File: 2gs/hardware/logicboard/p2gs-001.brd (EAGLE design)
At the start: 91 x 90 mm, 66 parts, among them J1 MKR, J10 1-Wire, J2 GPIO, J3 Vcc, J5 SPI, J6 LED, J7 DIN5, K1 G5V1, Q1 220mA/50V/3.5Ω, Q2 220mA/50V/3.5Ω, T1 2SC1815

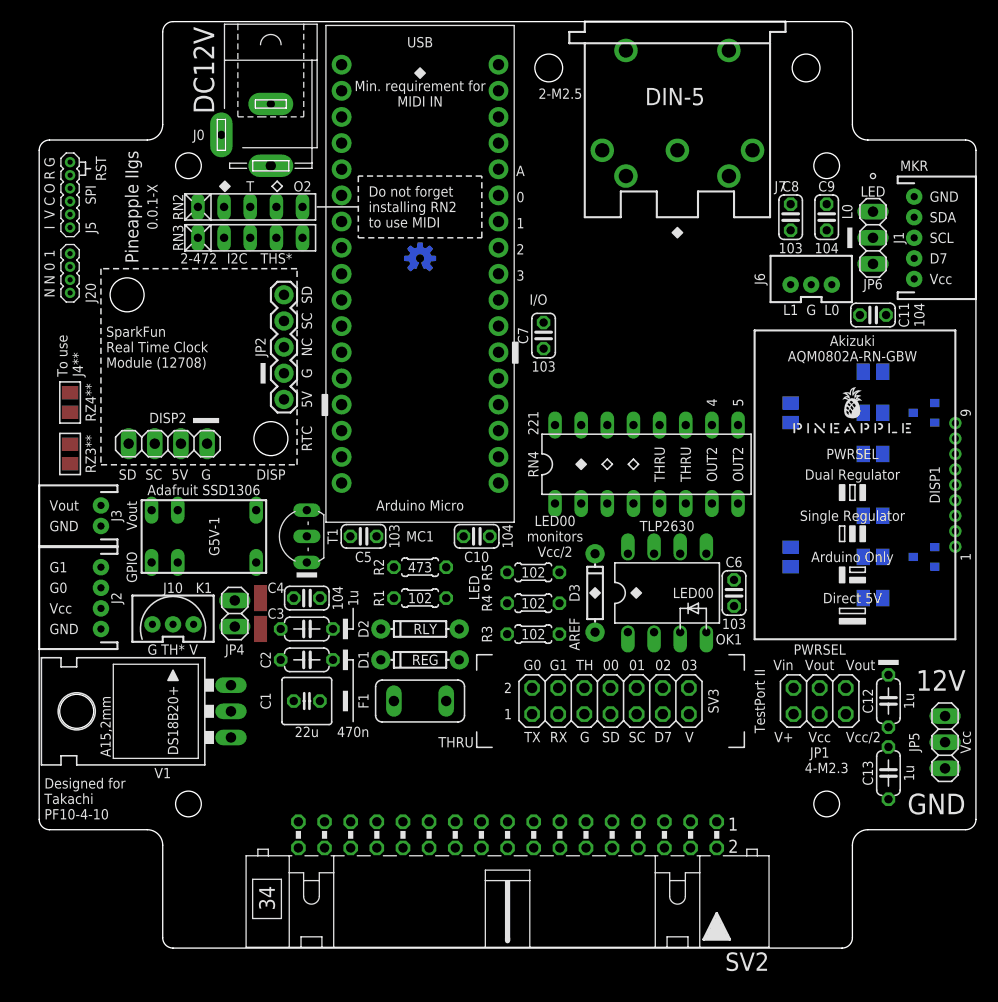
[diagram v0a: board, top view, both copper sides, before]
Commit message: Routed.
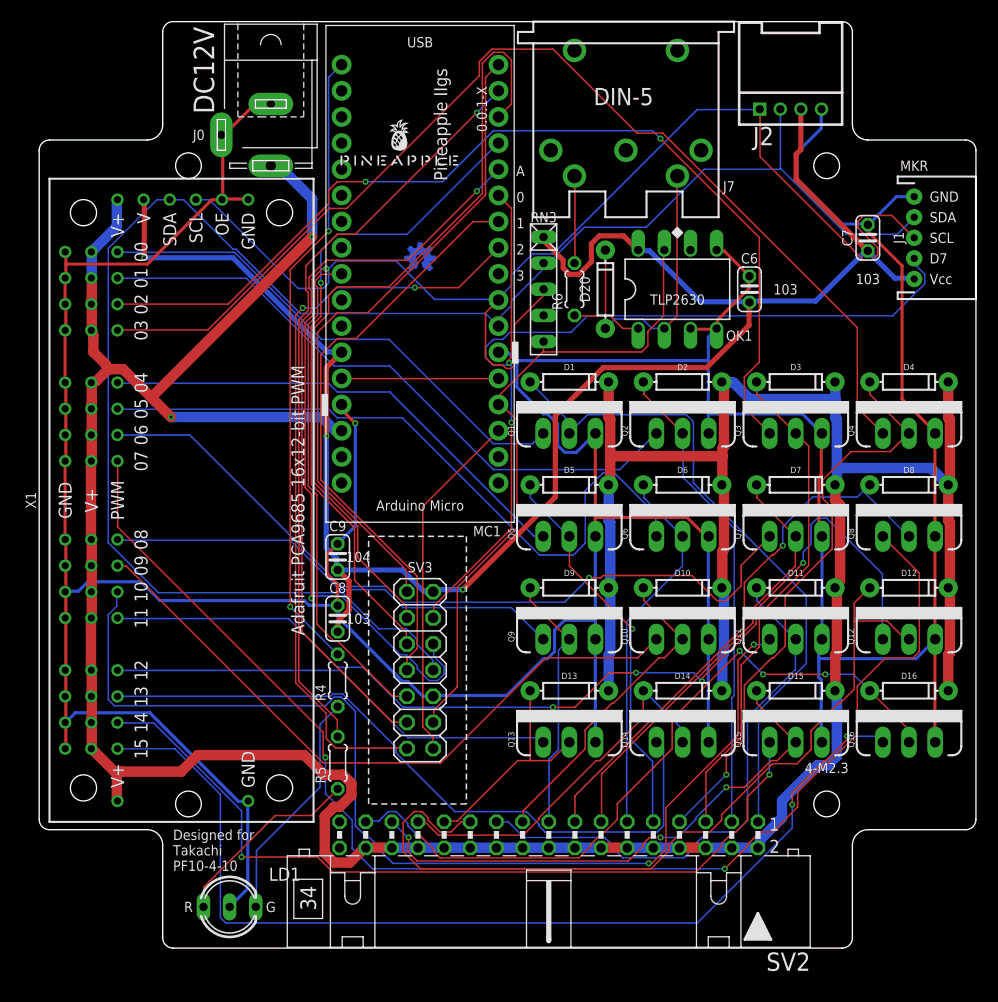
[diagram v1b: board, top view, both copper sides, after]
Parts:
- removed A, B: (no value), wirepad:SMD1,27-2,54
- removed C1: 22u, rcl:C025-050X050
- removed C10, C11, C4: 100n, rcl:C025-024X044
- removed C12, C13, C3: 1u, rcl:C050-024X044
- removed C2: 470n, rcl:C050-024X044
- removed C5: 10n, resistor:C025-024X044
- removed DISP1: AQM0802A-RN-GBW, AQM0802A-RN-GBW:AQM0802A-RN-GBW-FOOTPRINT
- removed DISP2: MNTR, pinhead:1X04
- removed F1: 1.8A, fuse:TE5
- removed H1, H2: STAND-OFF, SparkFun-Hardware:STAND-OFF
- removed J10: 1-Wire, SparkFun-Connectors:JST-3-PTH-VERT
- removed J20: (no value), SparkFun-Connectors:1X04_1.27MM
- removed J3: Vcc, SparkFun-Connectors:JST-2-PTH
- removed J5: SPI, SparkFun-Connectors:1X06_1.27MM
- removed J6: LED, SparkFun-Connectors:JST-3-PTH-VERT
- removed JP1: PWRSEL, pinhead:2X03
- removed JP2: RTC, SparkFun-Connectors:1X05
- removed JP4: RLYJMP, pinhead:1X02
- removed JP5: PWR, pinhead:1X03
- removed JP6: LED, pinhead:1X03
- removed K1: G5V1, relay:G5V1
- removed R1, R3: 1k, resistor:0204/5
- removed R101, R102, R103, R104: 10k, rcl:M2012
- removed R2: 47k, resistor:0204/5
- removed RN2: 4.7k, resistor-net:RN-5
- removed RN4: 220, resistor-dil:DIL16
- removed RZ1***, RZ2***, RZ3**, RZ4**, VCCBRIDGE***: Inf, rcl:M2012
- removed T1: 2SC1815, transistor:TO92-ECB
- removed V1: 5V, v-reg:78XXL
- removed VDDBRIDGE: 0, rcl:M2012
- added D10, D11, D12, D13, D14, D15, D16, D4, D5, D6, D7, D8, D9: 200mA/100V/1V, SparkFun-DiscreteSemi:DIODE-1N4148
- added D20: (no value), SparkFun-DiscreteSemi:DIODE-1N4148
- added LD1: Red/Green, led:DUOLED-C-5MM
- added Q10, Q11, Q12, Q13, Q14, Q15, Q16, Q3, Q4, Q5, Q6, Q7, Q8, Q9: 60V/32A/35mΩ, SparkFun-DiscreteSemi:TO220V
- added R6: 220, resistor:0204/5
- added X1: ADAFRUIT-PCA9685, adafruit-pca9685:ADAFRUIT-PCA9685-FOOTPRINT
- D1, D2, D3: value (none) -> 200mA/100V/1V
- J0: value (none) -> 12V
- J2: value GPIO -> (none); device SparkFun-Connectors:JST-4-PTH -> Connector:4P-2.0-90D
- Q1, Q2: value 220mA/50V/3.5Ω -> 60V/32A/35mΩ; device SparkFun-DiscreteSemi:SOT23-3 -> SparkFun-DiscreteSemi:TO220V
- R4, R5: value 1k -> 330
- SV2: value (none) -> LD
- moved J2 82.1 mm to (73.0, 81.5), turned to 0 degrees
- moved C8 58.8 mm to (29.0, 32.0)
- moved C9 57.8 mm to (29.0, 38.0)
- moved U$1 51.1 mm to (35.0, 76.0)
- moved Q1 36.5 mm to (51.5, 50.0), flipped to the top, turned to 0 degrees
- moved D2 35.0 mm to (62.5, 55.0), turned to 0 degrees
- moved C7 32.9 mm to (80.5, 69.0)
- moved D1 30.6 mm to (51.5, 55.0), turned to 0 degrees
- moved C6 29.5 mm to (69.0, 64.0)
- moved OK1 29.5 mm to (62.0, 64.0)
- moved RN3 28.9 mm to (49.0, 64.0), turned to 270 degrees
- moved D3 28.3 mm to (73.5, 55.0), turned to 0 degrees
- moved R5 26.5 mm to (29.0, 18.0), turned to 90 degrees
- moved Q2 23.6 mm to (62.5, 50.0), flipped to the top, turned to 0 degrees
- moved R4 20.4 mm to (29.0, 26.0), turned to 90 degrees
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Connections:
- removed net CAP1N: C12.2, DISP1.3
- removed net CAP1P: C12.1, DISP1.4
- removed net LCDVOUT: C13.2, DISP1.2
- removed net MNTRA: OK1.4, RN4.16
- removed net NMO2RTN: RN2.5
- removed net NMORTN: RN2.4
- removed net NMTRTN: RN2.3
- removed net RLYDRV: R1.1, R2.2, T1.B
- removed net RLYOUT: K1.10
- removed net RLYOUT1: RZ3**.2
- removed net RLYOUT2: RZ4**.2
- removed net RLYSNK: D2.A, K1.9, T1.C
- removed net SCL3V: DISP1.8, Q1.2, R102.1, RZ1***.2
- removed net SDA3V: DISP1.7, Q2.2, R104.1, RZ2***.2
- removed net V+: C1.1, C2.1, D1.C, J0.3, JP1.1, JP5.3, V1.IN
- removed net VCC/2: JP1.5, R3.2, RN4.1
- removed net VCC/VDD: C11.1, C13.1, DISP1.5, DISP1.9, VCCBRIDGE***.1, VDDBRIDGE.1
- removed net VOUT: F1.2, JP1.4, JP1.6
- removed net VOUTRAW: B.1, C3.1, C4.1, D1.A, J3.2, JP4.2, K1.5, K1.6, RZ3**.1, V1.OUT
- removed net VOUTRAW2: A.1, F1.1, JP4.1, K1.1, RZ4**.1
- new net LD00: D1.A, Q1.2, SV2.1
- new net LD01: D2.A, Q2.2, SV2.3
- new net LD02: D3.A, Q3.2, SV2.5
- new net LD03: D4.A, Q4.2, SV2.7
- new net LD04: D5.A, Q5.2, SV2.9
- new net LD05: D6.A, Q6.2, SV2.11
- new net LD06: D7.A, Q7.2, SV2.13
- new net LD07: D8.A, Q8.2, SV2.15
- new net LD08: D9.A, Q9.2, SV2.17
- new net LD09: D10.A, Q10.2, SV2.19
- new net LD10: D11.A, Q11.2, SV2.21
- new net LD11: D12.A, Q12.2, SV2.23
- new net LD12: D13.A, Q13.2, SV2.25
- new net LD13: D14.A, Q14.2, SV2.27
- new net LD14: D15.A, Q15.2, SV2.29
- new net LD15: D16.A, Q16.2, SV2.31
- new net PWM00: Q1.1, X1.PWM00
- new net PWM01: Q2.1, X1.PWM01
- new net PWM02: Q3.1, X1.PWM02
- new net PWM03: Q4.1, X1.PWM03
- new net PWM04: Q5.1, X1.PWM04
- new net PWM05: Q6.1, X1.PWM05
- new net PWM06: Q7.1, X1.PWM06
- new net PWM07: Q8.1, X1.PWM07
- new net PWM08: Q9.1, X1.PWM08
- new net PWM09: Q10.1, X1.PWM09
- new net PWM10: Q11.1, X1.PWM10
- new net PWM11: Q12.1, X1.PWM11
- new net PWM12: Q13.1, X1.PWM12
- new net PWM13: Q14.1, X1.PWM13
- new net PWM14: Q15.1, X1.PWM14
- new net PWM15: Q16.1, X1.PWM15
- net AREF: no longer C10.1, R3.1
- net GND: now also J2.4, LD1.C, OK1.4, Q1.3, Q10.3, Q11.3, Q12.3, Q13.3, Q14.3, Q15.3, Q16.3, Q2.3, Q3.3, Q4.3, Q5.3, Q6.3, Q7.3, Q8.3, Q9.3, X1.GND00, X1.GND01, X1.GND02, X1.GND03, X1.GND04, X1.GND05, X1.GND06, X1.GND07, X1.GND08, X1.GND09, X1.GND10, X1.GND11, X1.GND12, X1.GND13, X1.GND14, X1.GND15, X1.LGND, X1.LOE, X1.RGND; no longer C1.2, C10.2, C11.2, C2.2, C3.2, C4.2, C5.2, DISP1.6, DISP2.1, J10.1, J2.1, J3.1, J5.6, J6.2, JP2.2, JP5.1, JP6.2, R2.1, T1.E, V1.GND
- net GPIO0: no longer J2.3, J20.3
- net GPIO1: no longer J2.4, J20.4
- net LED0A: now also LD1.AR; no longer J6.3, JP6.3
- net LED1A: now also LD1.AX; no longer J6.1, JP6.1
- net MIDIINSND: now also D20.C, R6.1; no longer D3.C, RN4.2
- net MIRTN: now also D20.A; no longer D3.A
- net MISND: now also R6.2; no longer RN4.15
- net MISO: no longer J5.1
- net MNTR: no longer OK1.6, RN3.5
- net MOSI: no longer J5.4
- net RLY: no longer R1.2
- net RST: no longer J5.5
- net RX: now also RN3.5; no longer RN2.2
- net SCK: no longer J5.3
- net SCL: now also J2.1, X1.LSCL; no longer DISP2.3, JP2.4, Q1.3, R101.1, RZ1***.1
- net SDA: now also J2.2, X1.LSDA; no longer DISP2.4, JP2.5, Q2.3, R103.1, RZ2***.1
- net THS: no longer J10.2, RN3.4
- net VCC: now also J2.3, X1.LVCC; no longer C5.1, D2.C, DISP2.2, J10.3, J2.2, J5.2, JP1.3, JP2.1, JP5.2, K1.2, R101.2, R103.2, RN2.1, VCCBRIDGE***.2
- net VDD: no longer Q1.1, Q2.1, R102.2, R104.2, VDDBRIDGE.2
- net VIN: now also D1.C, D10.C, D11.C, D12.C, D13.C, D14.C, D15.C, D16.C, D2.C, D3.C, D4.C, D5.C, D6.C, D7.C, D8.C, D9.C, J0.3, SV2.10, SV2.12, SV2.14, SV2.16, SV2.18, SV2.2, SV2.20, SV2.22, SV2.24, SV2.26, SV2.28, SV2.30, SV2.32, SV2.4, SV2.6, SV2.8, X1.LV+, X1.RV+, X1.V+00, X1.V+01, X1.V+02, X1.V+03, X1.V+04, X1.V+05, X1.V+06, X1.V+07, X1.V+08, X1.V+09, X1.V+10, X1.V+11, X1.V+12, X1.V+13, X1.V+14, X1.V+15; no longer JP1.2
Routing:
- net GND: track 0.00 -> 448.4 mm, vias 0 -> 1
- net VIN: track 0.00 -> 369.6 mm, vias 0 -> 2
- net VCC: track 0.00 -> 179.8 mm, vias 0 -> 3
- net SCL: track 0.00 -> 173.3 mm, vias 0 -> 2
- net SDA: track 0.00 -> 168.2 mm
- net PWM07: track 0.00 -> 128.0 mm, vias 0 -> 2
- net PWM03: track 0.00 -> 106.5 mm
- net PWM10: track 0.00 -> 104.7 mm, vias 0 -> 2
- net PWM15: track 0.00 -> 98.3 mm, vias 0 -> 2
- net PWM11: track 0.00 -> 97.6 mm, vias 0 -> 4
- net D7GATE: track 0.00 -> 96.8 mm, vias 0 -> 2
- net PWM02: track 0.00 -> 95.0 mm, vias 0 -> 2
- net LD11: track 0.00 -> 81.2 mm
- net PWM14: track 0.00 -> 80.5 mm, vias 0 -> 2
- net DTCT2: track 0.00 -> 76.9 mm
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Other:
- board text removed: "00"
- board text removed: "01"
- board text removed: "02"
- board text removed: "03"
- board text removed: "102"
- board text removed: "12V"
- board text removed: "1u"
- board text removed: "2-472"
- board text removed: "2-M2.5"
- board text removed: "221"
- board text removed: "22u"
- board text removed: "4"
- board text removed: "470n"
- board text removed: "473"
- board text removed: "5"
- board text removed: "5V"
- board text removed: "9"
- board text removed: "AREF"
- board text removed: "Adafruit SSD1306"
- board text removed: "Akizuki AQM0802A-RN-GBW"
- board text removed: "Arduino Only"
- board text removed: "C"
- board text removed: "DISP"
- board text removed: "DS18B20+"
- board text removed: "Direct 5V"
- board text removed: "Do not forget installing RN2 to use MIDI"
- board text removed: "Dual Regulator"
- board text removed: "G0"
- board text removed: "G1"
- board text removed: "G5V-1"
- board text removed: "I"
- board text removed: "I/O"
- board text removed: "I2C"
- board text removed: "L0"
- board text removed: "L1"
- board text removed: "LED"
- board text removed: "LED00"
- board text removed: "LED00 monitors Vcc/2"
- board text removed: "Min. requirement for MIDI IN"
- board text removed: "N"
- board text removed: "NC"
- board text removed: "O"
- board text removed: "O2"
- board text removed: "OUT2"
- board text removed: "PWRSEL"
- board text removed: "REG"
- board text removed: "RST"
- board text removed: "RTC"
- board text removed: "RX"
- board text removed: "SC"
- board text removed: "SD"
- board text removed: "Single Regulator"
- board text removed: "SparkFun Real Time Clock Module (12708)"
- board text removed: "T"
- board text removed: "TH"
- board text removed: "TH*"
- board text removed: "THRU"
- board text removed: "TX"
- board text removed: "TestPort II"
- board text removed: "To use J4**"
- board text removed: "V"
